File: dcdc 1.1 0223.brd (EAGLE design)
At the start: 62.2 x 44.4 mm, 21 parts, among them M1 BSS97, X2 OUTPUT

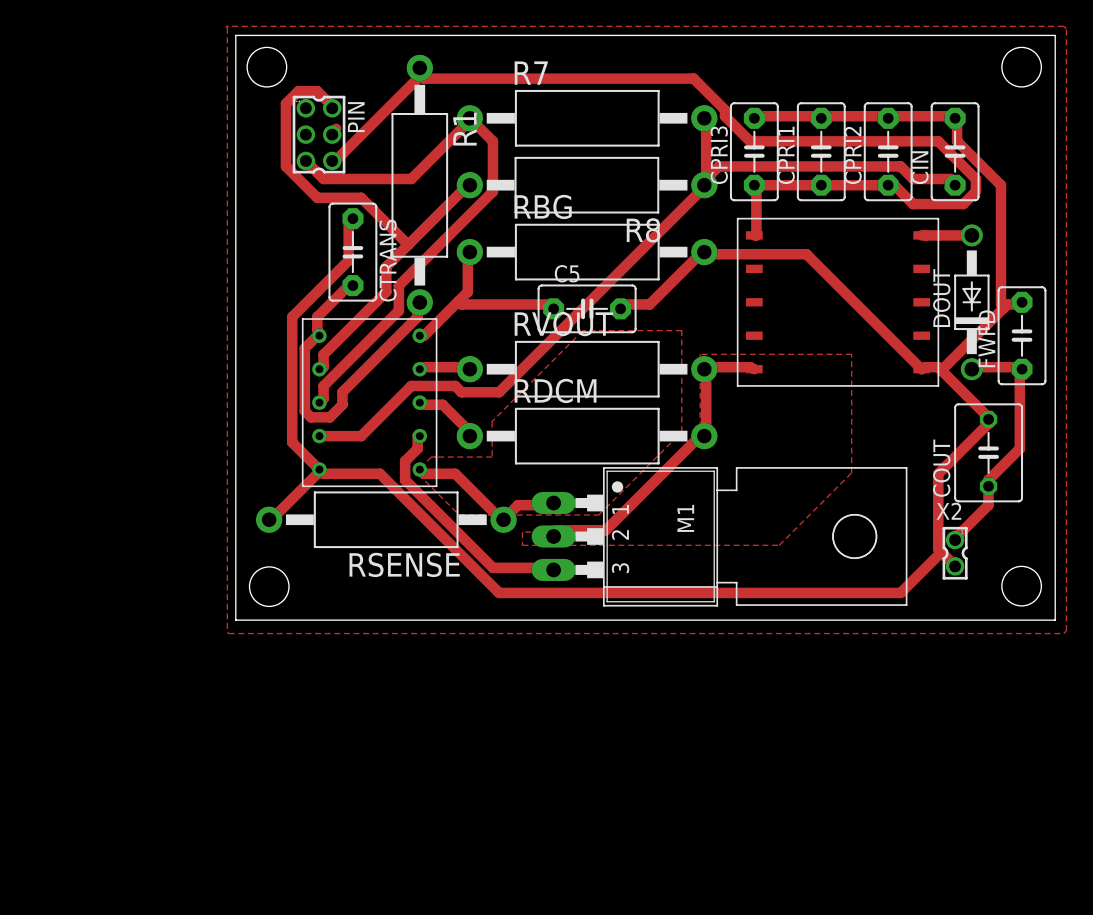
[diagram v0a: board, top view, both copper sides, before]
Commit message: second commit
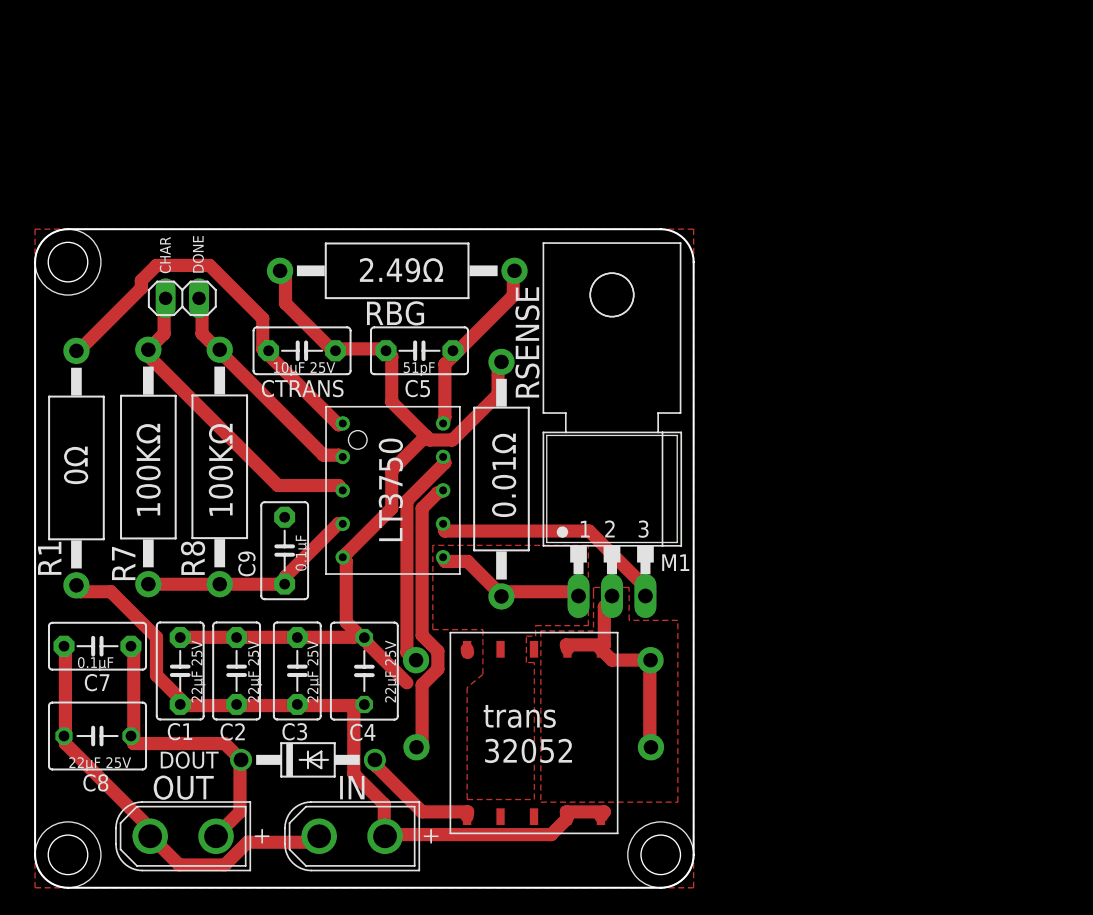
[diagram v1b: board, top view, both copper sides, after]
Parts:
- removed CIN, CPRI1, CPRI2, CPRI3, FWFD: (no value), capacitor-wima:C5B3.5
- removed COUT: (no value), rcl:C050-050X075
- removed PIN: Input, con-garry:332-06
- removed X2: OUTPUT, con-garry:332-02
- added C1, C2, C3, C7, C9: (no value), capacitor-wima:C5B3.5
- added C4, C8: (no value), rcl:C050-050X075
- added IN, OUT: XT30UPB-M, amass:XT30UPB-M
- added JP1: PINHD-1X2, Connector:1X02
- moved DOUT 61.2 mm to (20.7, 9.71), turned to 0 degrees
- moved R7 42.5 mm to (8.60, 31.9), turned to 270 degrees
- moved U$2 35.2 mm to (44.2, 4.13), turned to 90 degrees
- moved R8 35.1 mm to (14.0, 31.9), turned to 90 degrees
- moved R1 33.8 mm to (3.14, 31.9), turned to 90 degrees
- moved RDCM 24.0 mm to (37.9, 10.7), flipped to the bottom, turned to 180 degrees
- moved RVOUT 22.5 mm to (37.8, 17.3), flipped to the bottom, turned to 180 degrees
- moved RBG 14.5 mm to (27.5, 46.8), turned to 180 degrees
- moved C5 13.1 mm to (29.2, 40.8), turned to 180 degrees
- moved RSENSE 9.27 mm to (35.4, 31.0), turned to 90 degrees
- moved CTRANS 8.43 mm to (20.3, 40.8), turned to 180 degrees
- moved U$1 6.89 mm to (23.4, 22.6)
- moved M1 0.86 mm to (43.8, 27.2), turned to 0 degrees
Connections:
- net 66 renamed SOURCE
- removed net N$15: PIN.5, R7.1, U$1.P$3
- removed net N$9: DOUT.A, U$2.P$6
- new net N$5: JP1.1, R7.1, U$1.P$3
- new net N$7: DOUT.A, U$2.P$1
- net 0: now also C1.2, C2.2, C3.2, C4.2, C7.2, C8.2, C9.2, IN.-, OUT.-, U$2.P$6; no longer CIN.2, COUT.2, CPRI1.2, CPRI2.2, CPRI3.2, FWFD.2, PIN.4, U$2.P$10, X2.2
- net DRAIN: now also U$2.P$10, U$2.P$9; no longer U$2.P$5
- net N$1: now also C9.1; no longer CIN.1
- net N$10: now also C7.1, C8.1, OUT.+; no longer COUT.1, FWFD.1, X2.1
- net N$13: now also C1.1, C2.1, C3.1, C4.1, IN.+, U$2.P$4, U$2.P$5; no longer CPRI1.1, CPRI2.1, CPRI3.1, PIN.6, U$2.P$1
- net N$8: now also JP1.2; no longer PIN.2
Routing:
- net 0: track 168.7 -> 99.1 mm
- net N$1: track 63.3 -> 16.9 mm
- net N$15: track 42.8 -> 0.00 mm
- net N$5: track 0.00 -> 23.9 mm
- net N$8: track 39.9 -> 17.3 mm
- net N$13: track 79.1 -> 56.7 mm
- net N$4: track 4.97 -> 21.5 mm
- net N$3: track 3.90 -> 17.0 mm
- net N$7: track 0.00 -> 9.22 mm
- net DRAIN: track 23.8 -> 18.3 mm
- net N$14: track 25.1 -> 29.7 mm
- net N$10: track 18.9 -> 22.9 mm
- net N$9: track 3.81 -> 0.00 mm
- net N$2: track 15.6 -> 14.0 mm
- net N$6: track 18.0 -> 18.5 mm
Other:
- board size 62.2 x 44.4 mm -> 50 x 50 mm
- board text added: "0.01Ω"
- board text added: "0.1μF"
- board text added: "0Ω"
- board text added: "100KΩ"
- board text added: "10μF 25V"
- board text added: "2.49Ω"
- board text added: "22μF 25V"
- board text added: "40.2KΩ"
- board text added: "51pF"
- board text added: "60.4KΩ"
- board text added: "CHAR"
- board text added: "DONE"
- board text added: "LT3750"
- board text added: "Ri-one SSL DC-DC conveter Ver 1.1 Feb 23,2023 Designed by Kotaro Ochiishi"
- board text added: "trans 32052"
